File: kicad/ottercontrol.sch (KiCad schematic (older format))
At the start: 79 parts, among them IC1 MAX485, IC2 USBLC6-4, IC3 USBLC6-2SC6, J1 USB_B_Micro, P1 Conn_01x02, Q1 Q_PMOS_GSD, U1 STM32F303CBT6, U2 MAX3051, U6 XL7015, U7 ACT4088, U8 MIC5504-3.3YM5, X1 programmer, X2 Conn_01x08, X3 Conn_01x05, Y1 16MHz

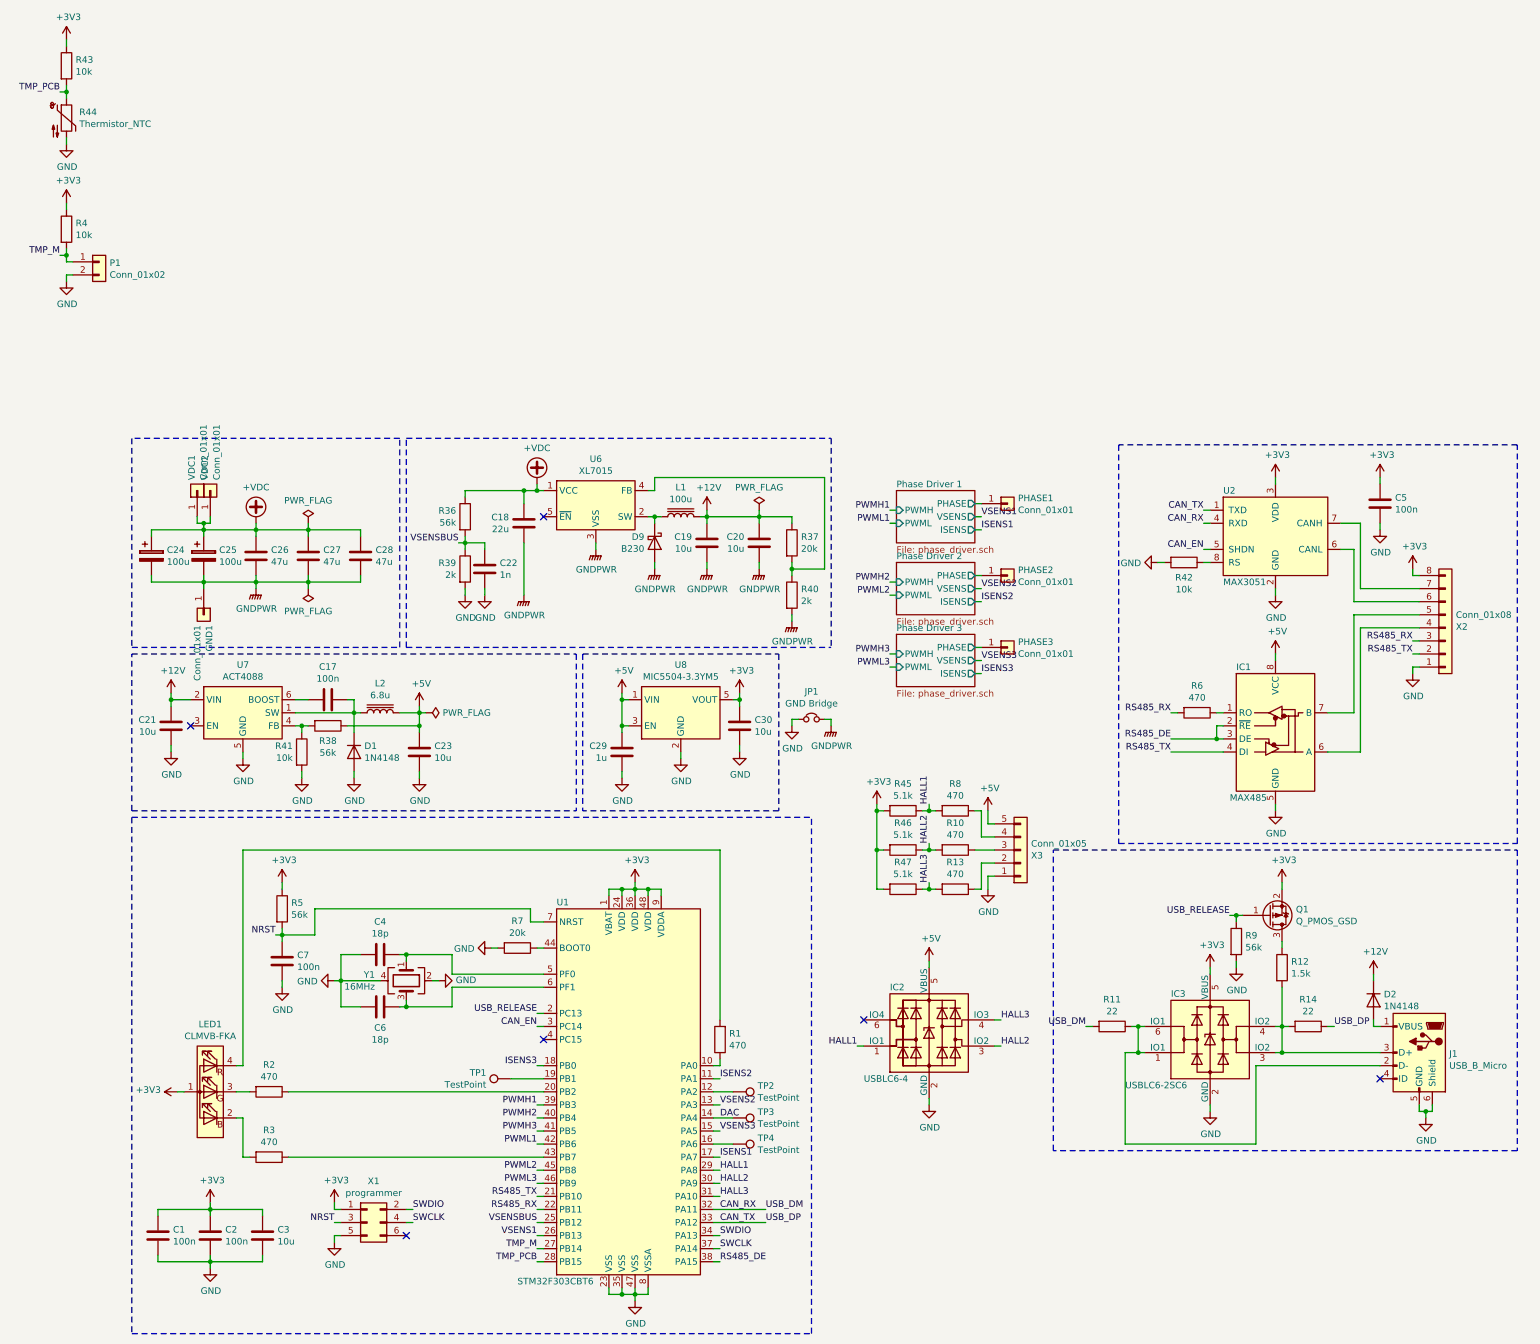
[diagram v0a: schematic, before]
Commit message: added finished adding MPNs to all components
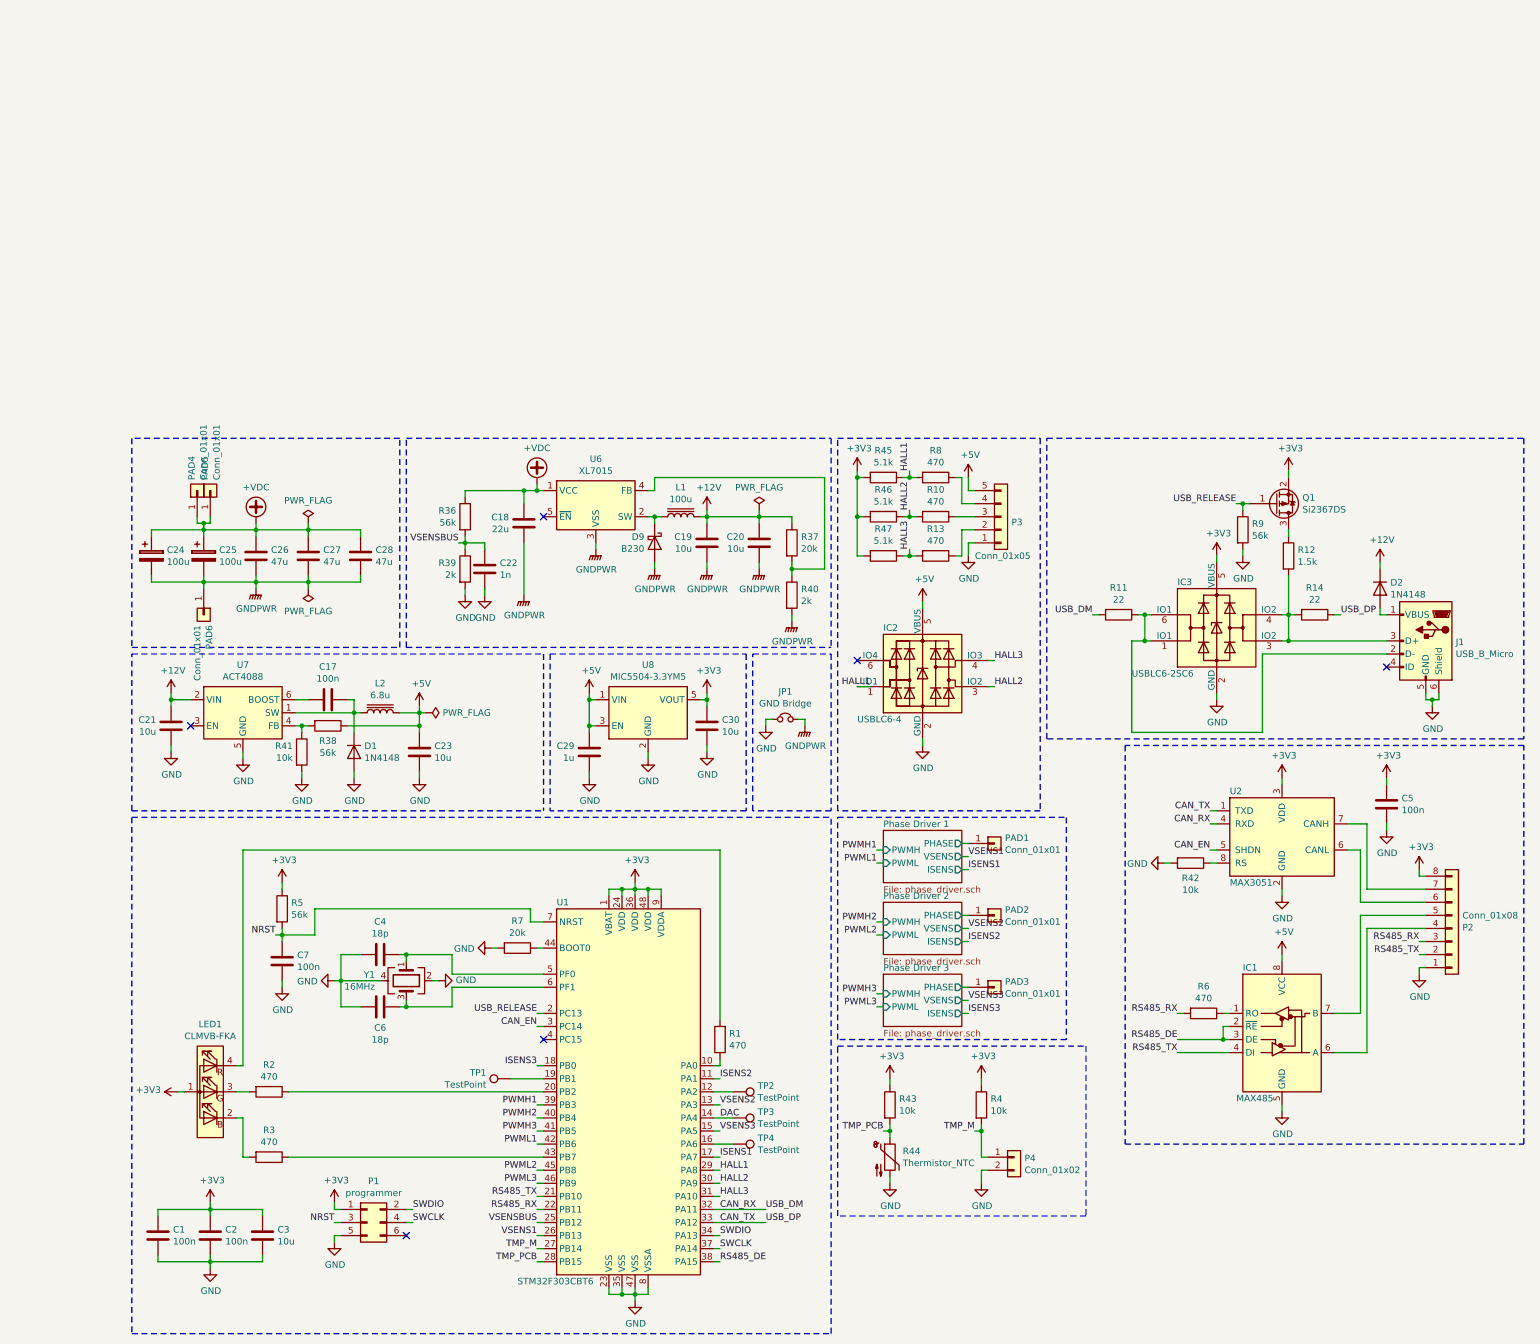
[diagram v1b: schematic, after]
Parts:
- C29: Voltage Rating DC 10 -> 25
- J1: MPN (none) -> 105017-0001
- JP1, TP1, TP2, TP3, TP4: MPN (none) -> n/a
- P1: renamed from X1; MPN (none) -> TC2030-MCP-NL
- P2: renamed from X2; MPN (none) -> 53261-0871
- P3: renamed from X3; MPN (none) -> 53261-0571
- P4: renamed from P1; MPN (none) -> n/a
- PAD1: renamed from PHASE1; MPN (none) -> n/a
- PAD2: renamed from PHASE2; MPN (none) -> n/a
- PAD3: renamed from PHASE3; MPN (none) -> n/a
- PAD4: renamed from VDC1; MPN (none) -> n/a
- PAD5: renamed from VDC2; MPN (none) -> n/a
- PAD6: renamed from GND1; MPN (none) -> n/a
- Q1: value Q_PMOS_GSD -> Si2367DS; MPN (none) -> SI2367DS-T1-GE3
- R1, R10, R13, R2, R3, R6, R8: MPN RC0603FR-07470RL -> RC0603FR-07100RL
- Y1: footprint Crystal:Crystal_SMD_5032-4Pin_5.0x3.2mm -> Crystal:Crystal_SMD_3225-4Pin_3.2x2.5mm; MPN (none) -> FA-238 16.0000MB-K3
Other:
- moved on the sheet: C29, C30, C5, D2, IC1, IC2, IC3, J1, JP1, P2, P3, P4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
